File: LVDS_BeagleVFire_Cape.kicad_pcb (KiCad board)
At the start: 2 copper layers, 80.5 x 94.5 mm, 52 parts, among them J1 Conn_02x16, J10 Conn_Coaxial_Small, J11 Conn_Coaxial_Small, J12 Conn_Coaxial_Small, J2 Conn_02x16, J3 RJHSE508002, J4 Conn_Coaxial_Small, J5 Conn_Coaxial_Small, J6 Conn_Coaxial_Small, J7 Conn_Coaxial_Small, J8 Conn_01x06_Pin, J9 Conn_Coaxial_Small, P1 BeagleBone_Black_Header, P2 BeagleBone_Black_Header, U1 SN65LVDT348D, U10 SN65MLVD206BD, U11 SN65MLVD206BD, U12 SN65MLVD206BD, U13 SN65LVDT348D, U2 SN65LVDT348D, U3 SN65LVDT348D, U4 SN65LVDT348D, U5 SN65LVDT348D, U6 SN65LVDT348D, U7 SN65LVDT348D, U8 SN65LVDT348D, U9 SN65MLVD206BD

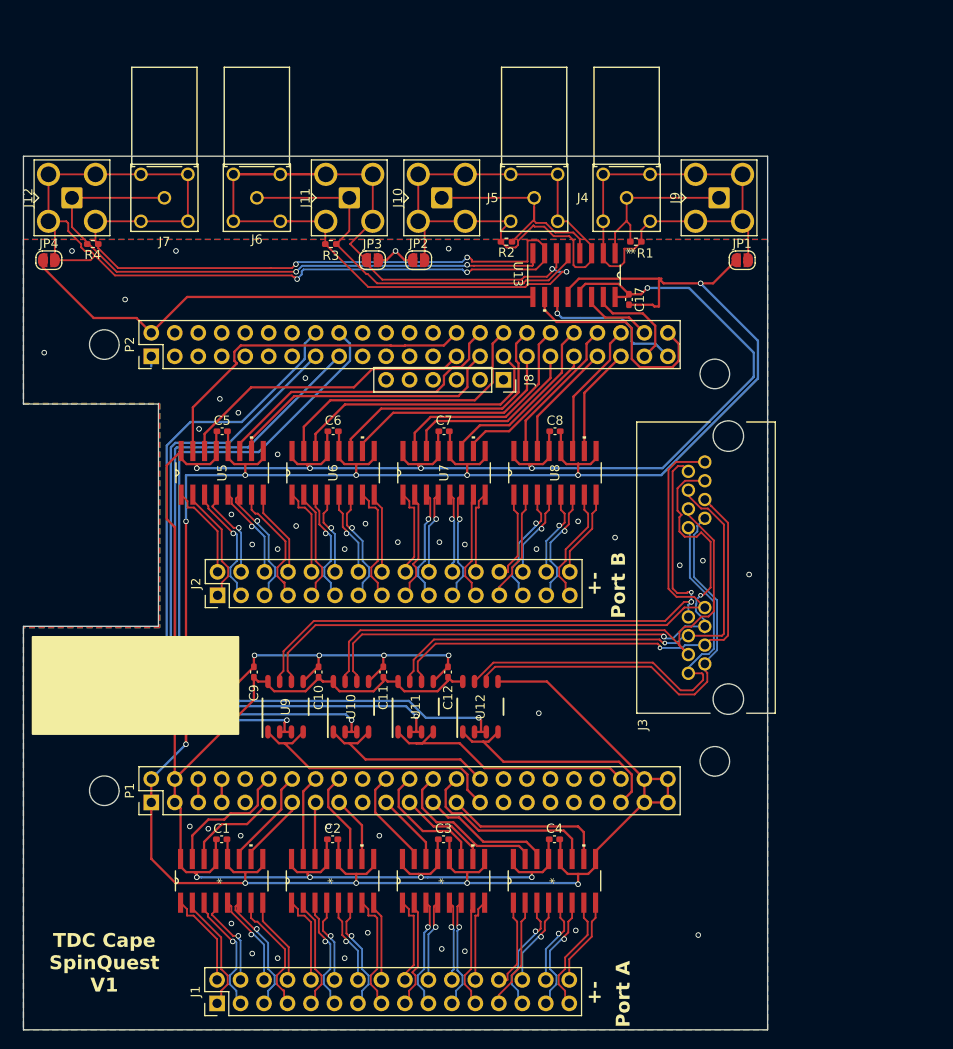
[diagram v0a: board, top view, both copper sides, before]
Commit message: v2
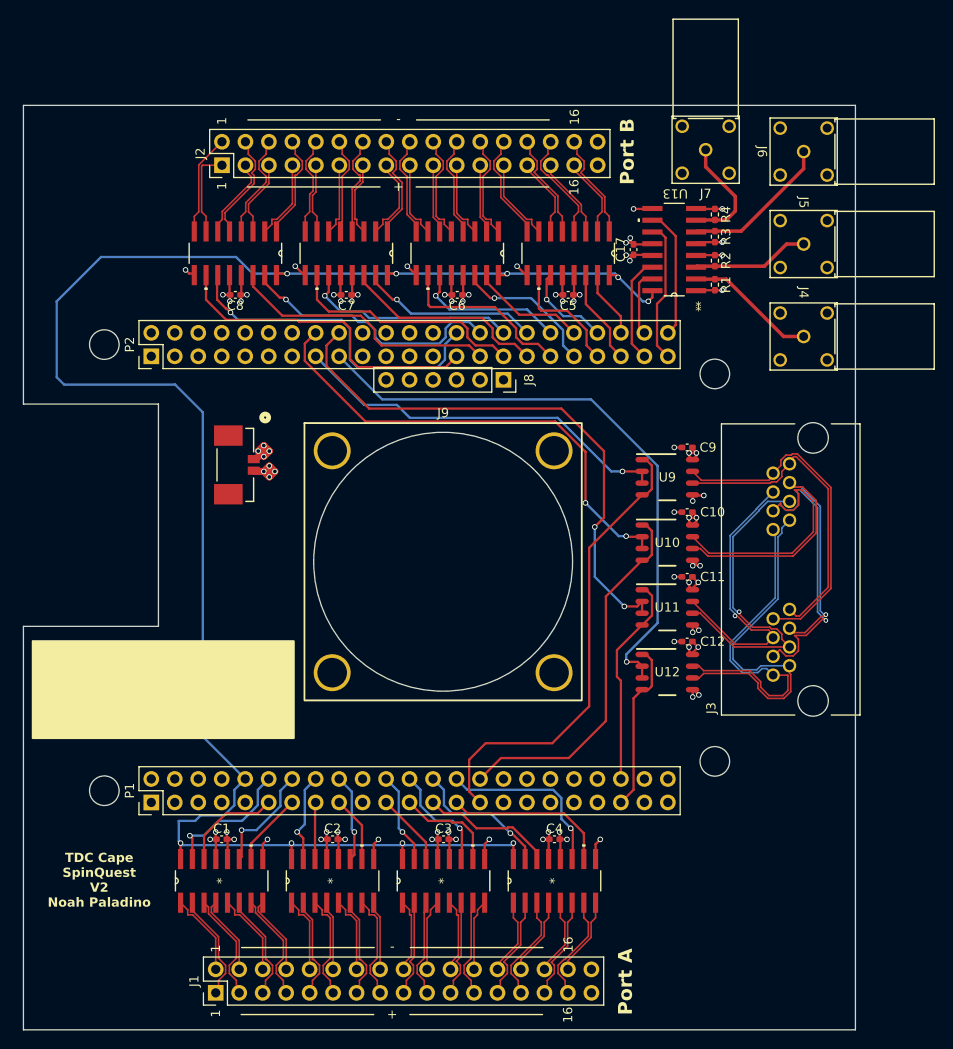
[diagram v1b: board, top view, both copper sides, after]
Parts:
- removed J10, J11, J12: Conn_Coaxial_Small, Connector_Coaxial:SMA_Amphenol_901-143_Horizontal
- removed JP1, JP2, JP3, JP4: SolderJumper_2_Open, Jumper:SolderJumper-2_P1.3mm_Open_RoundedPad1.0x1.5mm
- J1, J2: footprint Connector_PinHeader_2.54mm:PinHeader_2x16_P2.54mm_Vertical -> Kria_Board_Parts:PinHeader_2x17_P2.54mm_Vertical_ECL
- J9: value Conn_Coaxial_Small -> ~; footprint Connector_Coaxial:SMA_Amphenol_901-143_Horizontal -> Kria_Board_Parts:LD3007MS_FAN
- moved R4 67.4 mm to (124.8, 61.8), turned to 90 degrees
- moved J6 59.4 mm to (134.4, 55.0), turned to -90 degrees
- moved J7 58.8 mm to (123.8, 54.8)
- moved C9 52.8 mm to (121.8, 87.0), turned to 180 degrees
- moved J9 49.4 mm to (95.4, 99.4)
- moved U9 48.2 mm to (119.7, 90.2), turned to 0 degrees
- moved J2 46.5 mm to (71.5, 56.5)
- moved U5 44.3 mm to (108.9, 66.0), turned to -90 degrees
- moved C10 43.5 mm to (121.8, 94.0), turned to 180 degrees
- moved U8 41.9 mm to (72.9, 66.0), turned to -90 degrees
- moved R3 41.6 mm to (124.8, 64.2), turned to -90 degrees
- moved C5 40.2 mm to (108.9, 70.5), turned to 180 degrees
- moved U10 38.5 mm to (119.7, 97.3), turned to 0 degrees
- moved C8 37.6 mm to (72.9, 70.5), turned to 180 degrees
- moved C11 34.4 mm to (121.8, 101.0), turned to 180 degrees
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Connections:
- J2 pad 1: /Discriminator Inputs/Port B/In0+ -> /Discriminator Inputs/Port B/In15+
- J2 pad 10: /Discriminator Inputs/Port B/In4- -> /Discriminator Inputs/Port B/In11-
- J2 pad 11: /Discriminator Inputs/Port B/In5+ -> /Discriminator Inputs/Port B/In10+
- J2 pad 12: /Discriminator Inputs/Port B/In5- -> /Discriminator Inputs/Port B/In10-
- J2 pad 13: /Discriminator Inputs/Port B/In6+ -> /Discriminator Inputs/Port B/In9+
- J2 pad 14: /Discriminator Inputs/Port B/In6- -> /Discriminator Inputs/Port B/In9-
- J2 pad 15: /Discriminator Inputs/Port B/In7+ -> /Discriminator Inputs/Port B/In8+
- J2 pad 16: /Discriminator Inputs/Port B/In7- -> /Discriminator Inputs/Port B/In8-
- J2 pad 17: /Discriminator Inputs/Port B/In8+ -> /Discriminator Inputs/Port B/In7+
- J2 pad 18: /Discriminator Inputs/Port B/In8- -> /Discriminator Inputs/Port B/In7-
- J2 pad 19: /Discriminator Inputs/Port B/In9+ -> /Discriminator Inputs/Port B/In6+
- J2 pad 2: /Discriminator Inputs/Port B/In0- -> /Discriminator Inputs/Port B/In15-
- J2 pad 20: /Discriminator Inputs/Port B/In9- -> /Discriminator Inputs/Port B/In6-
- J2 pad 21: /Discriminator Inputs/Port B/In10+ -> /Discriminator Inputs/Port B/In5+
- J2 pad 22: /Discriminator Inputs/Port B/In10- -> /Discriminator Inputs/Port B/In5-
- J2 pad 23: /Discriminator Inputs/Port B/In11+ -> /Discriminator Inputs/Port B/In4+
- J2 pad 24: /Discriminator Inputs/Port B/In11- -> /Discriminator Inputs/Port B/In4-
- J2 pad 25: /Discriminator Inputs/Port B/In12+ -> /Discriminator Inputs/Port B/In3+
- J2 pad 26: /Discriminator Inputs/Port B/In12- -> /Discriminator Inputs/Port B/In3-
- J2 pad 27: /Discriminator Inputs/Port B/In13+ -> /Discriminator Inputs/Port B/In2+
- J2 pad 28: /Discriminator Inputs/Port B/In13- -> /Discriminator Inputs/Port B/In2-
- J2 pad 29: /Discriminator Inputs/Port B/In14+ -> /Discriminator Inputs/Port B/In1+
- J2 pad 3: /Discriminator Inputs/Port B/In1+ -> /Discriminator Inputs/Port B/In14+
- J2 pad 30: /Discriminator Inputs/Port B/In14- -> /Discriminator Inputs/Port B/In1-
- J2 pad 31: /Discriminator Inputs/Port B/In15+ -> /Discriminator Inputs/Port B/In0+
- J2 pad 32: /Discriminator Inputs/Port B/In15- -> /Discriminator Inputs/Port B/In0-
- J2 pad 4: /Discriminator Inputs/Port B/In1- -> /Discriminator Inputs/Port B/In14-
- J2 pad 5: /Discriminator Inputs/Port B/In2+ -> /Discriminator Inputs/Port B/In13+
- J2 pad 6: /Discriminator Inputs/Port B/In2- -> /Discriminator Inputs/Port B/In13-
- J2 pad 7: /Discriminator Inputs/Port B/In3+ -> /Discriminator Inputs/Port B/In12+
- J2 pad 8: /Discriminator Inputs/Port B/In3- -> /Discriminator Inputs/Port B/In12-
- J2 pad 9: /Discriminator Inputs/Port B/In4+ -> /Discriminator Inputs/Port B/In11+
- J4 pad 1: /Trigger Interface/NIM1- -> /Trigger Interface/NIM1+
- J4 pad 2: /Trigger Interface/NIM1+ -> GND
- J5 pad 1: /Trigger Interface/NIM2- -> /Trigger Interface/NIM2+
- J5 pad 2: /Trigger Interface/NIM2+ -> GND
- J6 pad 1: /Trigger Interface/NIM3- -> /Trigger Interface/NIM3+
- J6 pad 2: /Trigger Interface/NIM3+ -> GND
- J7 pad 1: /Trigger Interface/NIM4- -> /Trigger Interface/NIM4+
- J7 pad 2: /Trigger Interface/NIM4+ -> GND
- J9 pad 1: /Trigger Interface/NIM1- -> GND
- J9 pad 2: /Trigger Interface/NIM1+ -> +5V
- P1 pad 10: /~{SYS_RESET} -> ~{SYS_RESET}
- P2 pad 15: /TS_BUS_SEL1 -> /TS_BUS_SEL0
- P2 pad 16: /TS_BUS_SEL0 -> /TS_BUS_SEL1
- P2 pad 17: /TS_BUS_SEL2 -> /TS_BUS_SEL3
- P2 pad 18: /TS_BUS_SEL3 -> /TS_BUS_SEL2
- P2 pad 27: /D17 -> /D16
- P2 pad 28: /D16 -> /D17
- P2 pad 29: /D19 -> /D18
- P2 pad 30: /D18 -> /D19
- P2 pad 31: /D21 -> /D20
- P2 pad 32: /D20 -> /D21
- P2 pad 33: /D23 -> /D22
- P2 pad 34: /D22 -> /D23
- P2 pad 35: /D25 -> /D24
- P2 pad 36: /D24 -> /D25
- P2 pad 37: /D27 -> /D26
- P2 pad 38: /D26 -> /D27
- P2 pad 39: /D29 -> /D28
- P2 pad 40: /D28 -> /D29
- P2 pad 41: /D31 -> /D30
- P2 pad 42: /D30 -> /D31
- P2 pad 43: /NIM0 -> /NIM1
- P2 pad 44: /NIM1 -> /NIM0
- R1 pad 1: /Trigger Interface/NIM1- -> GND
- R2 pad 1: /Trigger Interface/NIM2- -> GND
- R3 pad 2: /Trigger Interface/NIM3- -> GND
- R4 pad 2: /Trigger Interface/NIM4- -> GND
- U1 pad 16: +3V3 -> ~{SYS_RESET}
- U13 pad 1: /Trigger Interface/NIM1- -> GND
- U13 pad 16: +3V3 -> ~{SYS_RESET}
- U13 pad 4: /Trigger Interface/NIM2- -> GND
- U13 pad 5: /Trigger Interface/NIM3- -> GND
- U13 pad 8: /Trigger Interface/NIM4- -> GND
- U2 pad 16: +3V3 -> ~{SYS_RESET}
- U3 pad 16: +3V3 -> ~{SYS_RESET}
- U4 pad 16: +3V3 -> ~{SYS_RESET}
- U5 pad 10: /D19 -> /D28
- U5 pad 11: /D18 -> /D29
- U5 pad 14: /D17 -> /D30
- U5 pad 15: /D16 -> /D31
- U5 pad 16: +3V3 -> ~{SYS_RESET}
- U6 pad 10: /D23 -> /D24
- U6 pad 11: /D22 -> /D25
- U6 pad 14: /D21 -> /D26
- U6 pad 15: /D20 -> /D27
- U6 pad 16: +3V3 -> ~{SYS_RESET}
- U7 pad 10: /D27 -> /D20
- U7 pad 11: /D26 -> /D21
- U7 pad 14: /D25 -> /D22
- U7 pad 15: /D24 -> /D23
- U7 pad 16: +3V3 -> ~{SYS_RESET}
- U8 pad 10: /D31 -> /D16
- U8 pad 11: /D30 -> /D17
- U8 pad 14: /D29 -> /D18
- U8 pad 15: /D28 -> /D19
- U8 pad 16: +3V3 -> ~{SYS_RESET}
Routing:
- net GND: track 417.3 -> 85.6 mm, vias 56 -> 47
- net +3V3: track 285.6 -> 49.4 mm, vias 9 -> 26
- net ~{SYS_RESET}: track 0.00 -> 196.8 mm, vias 0 -> 9
- net /Trigger Interface/NIM4+: track 159.6 -> 12.6 mm, vias 4 -> 0
- net /Trigger Interface/NIM3+: track 109.3 -> 16.2 mm, vias 2 -> 0
- net /Trigger Interface/NIM4-: track 66.7 -> 0.00 mm, vias 2 -> 0
- net /Trigger Interface/NIM2+: track 63.8 -> 12.7 mm
- net /Trigger Interface/NIM3-: track 44.3 -> 0.00 mm
- net +5V: track 2.54 -> 45.6 mm, vias 0 -> 4
- net /Trigger Interface/NIM1+: track 52.8 -> 14.2 mm
- net /Trigger Interface/D1+: track 72.4 -> 33.9 mm
- net /Trigger Interface/D1-: track 69.7 -> 36.8 mm, vias 2 -> 0
- net /Trigger Interface/NIM2-: track 24.5 -> 0.00 mm
- net /Trigger Interface/D2+: track 67.1 -> 43.3 mm, vias 2 -> 1
- net /Trigger Interface/D3-: track 55.1 -> 32.1 mm
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- added copper zone on In2.Cu, net +3V3
- added copper zone on In1.Cu, net GND
- removed copper zone on B.Cu, net GND
- removed copper zone on F.Cu, net GND
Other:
- board size 80.5 x 94.5 mm -> 90 x 100 mm
- copper layers 2 -> 4
- board text added: "TDC Cape SpinQuest V2 Noah Paladino"
- board text removed: "+-"
- board text removed: "TDC Cape SpinQuest V1"
